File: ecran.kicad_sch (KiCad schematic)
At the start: 15 parts, among them J6 MEC1-110-02-F-D-A, J8 MEC1-110-02-F-D-A, SW1 RotaryEncoder_Switch_MP

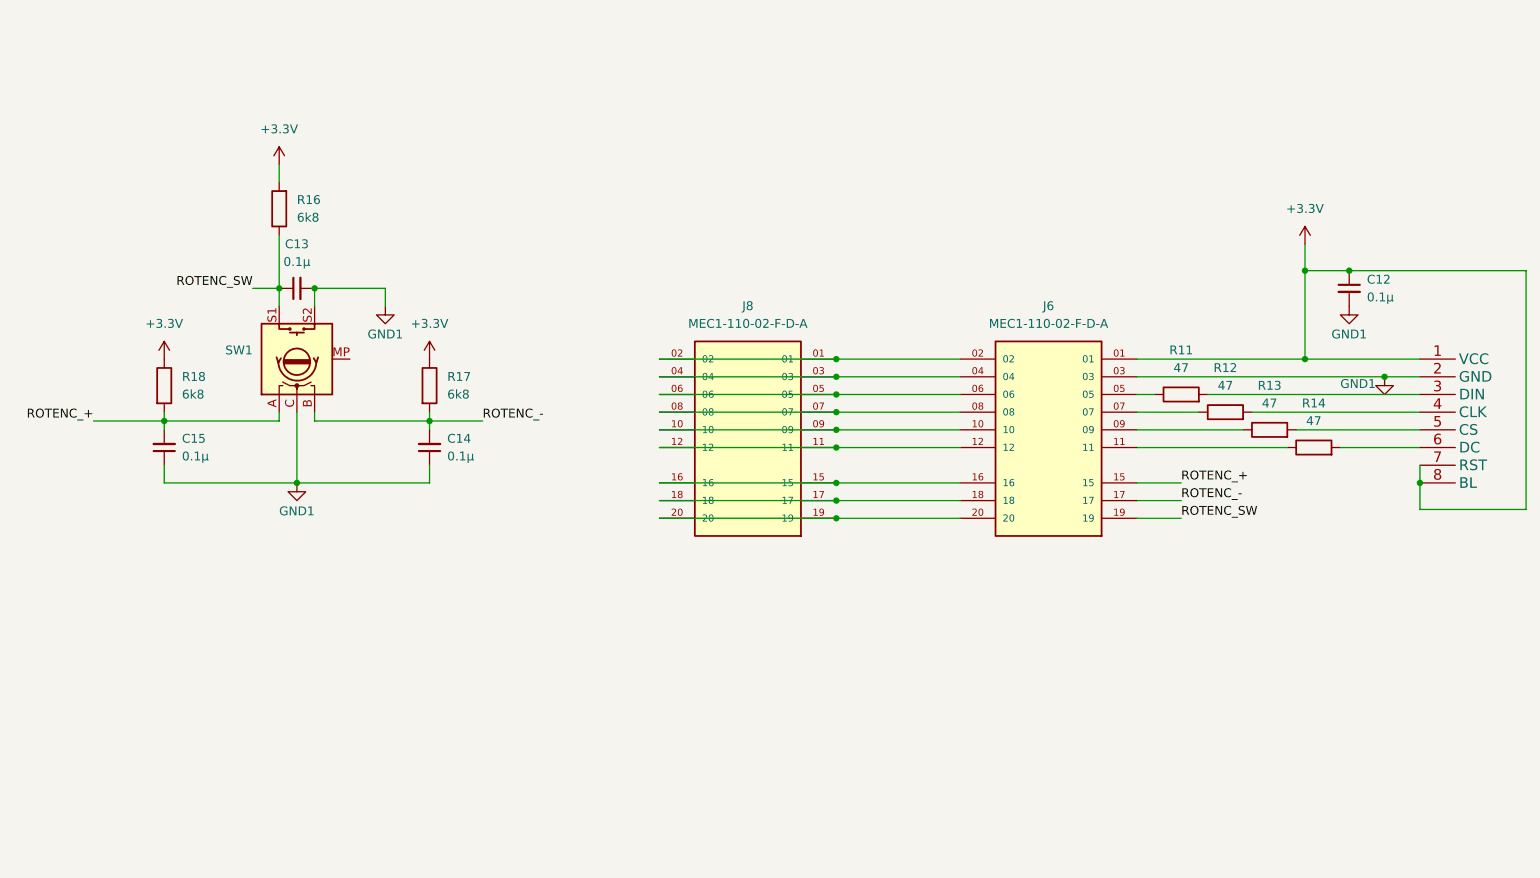
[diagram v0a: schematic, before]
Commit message: maj puissance
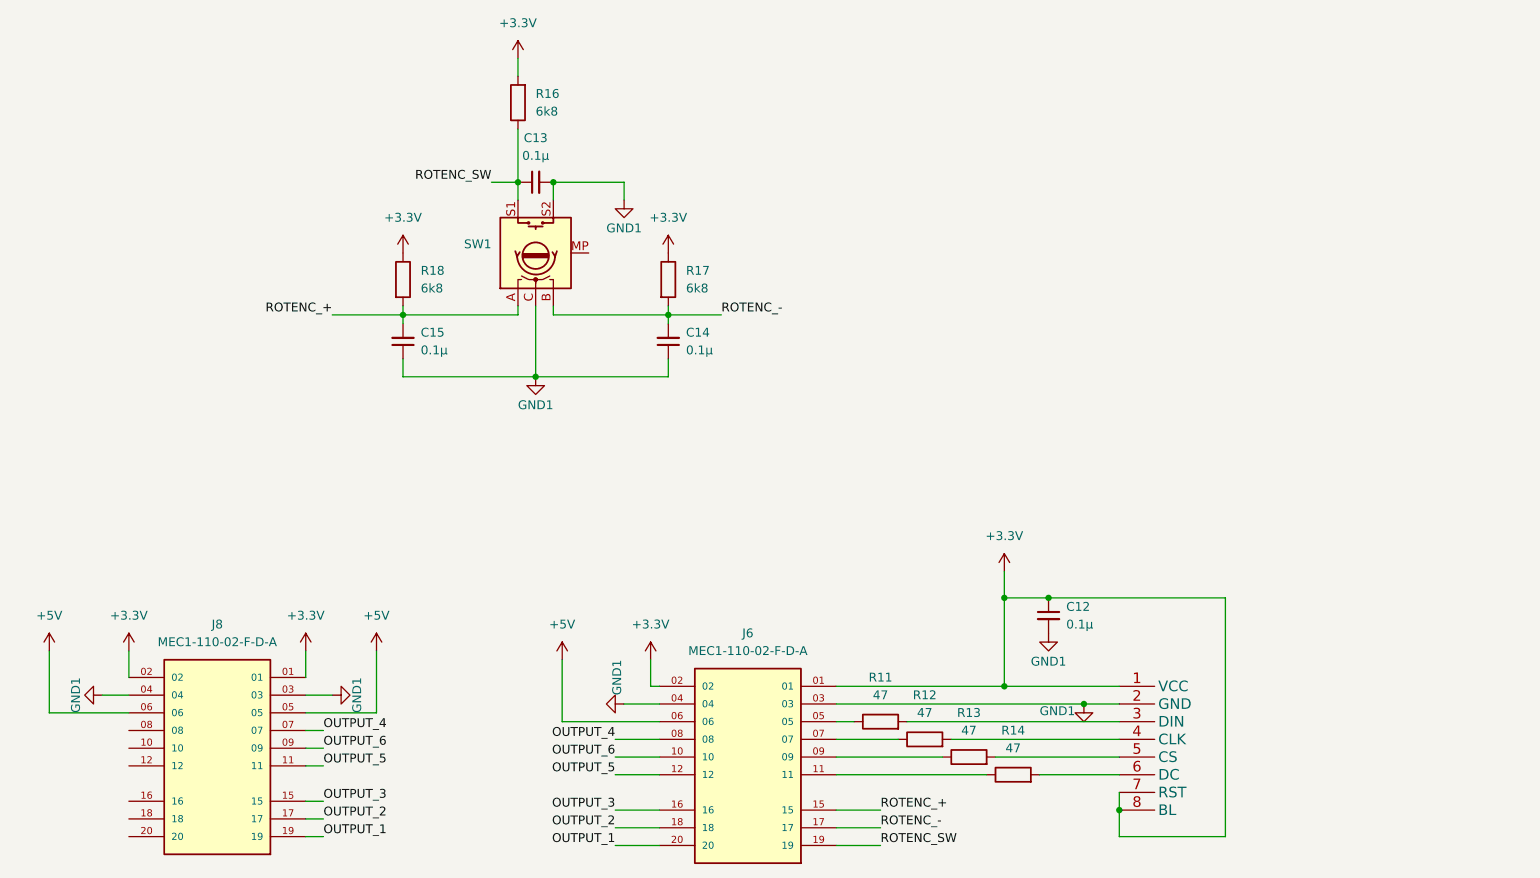
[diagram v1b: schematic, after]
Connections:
- net +3.3V: now also J6.02, J8.01, J8.02
- net GND1: now also J6.04, J8.03, J8.04
- net +5V: now reaches J6.06, J8.05, J8.06
- net OUTPUT_4: now reaches J6.08, J8.07
- net OUTPUT_4: no longer J8.08
- net OUTPUT_6: now reaches J6.10, J8.09
- net OUTPUT_6: no longer J8.10
- net OUTPUT_5: now reaches J6.12, J8.11
- net OUTPUT_5: no longer J8.12
- net OUTPUT_3: now reaches J6.16, J8.15
- net OUTPUT_3: no longer J8.16
- net OUTPUT_2: now reaches J6.18, J8.17
- net OUTPUT_2: no longer J8.18
- net OUTPUT_1: now reaches J6.20, J8.19
- net OUTPUT_1: no longer J8.20
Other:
- moved on the sheet: C12, C13, C14, C15, J6, J8, R11, R12, R13, R14, R16, R17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
